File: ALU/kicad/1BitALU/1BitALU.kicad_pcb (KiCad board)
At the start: 2 copper layers, 165.1 x 165.1 mm, 55 parts, among them P1 CONN_6, P2 CONN_2, P3 Power, U1 xor3a, U10 and3a, U11 or2a, U12 and3b, U13 inv3b, U14 and3c, U15 or3a, U16 xor1b, U17 xor1a, U18 xor2b, U19 and4a, U2 and2a, U20 xor2a, U21 and4b, U22 and4c, U23 or3b, U24 and5a, U25 and5b, U26 inv5c, U27 and5c, U28 or3c, U29 and6a, U3 xor3b, U30 inv6b, U31 and6b, U32 inv6c, U33 and6c, U34 or3d, U4 and2b, U5 or1b, U6 and1a, U7 and1b, U8 or1a, U9 or2b

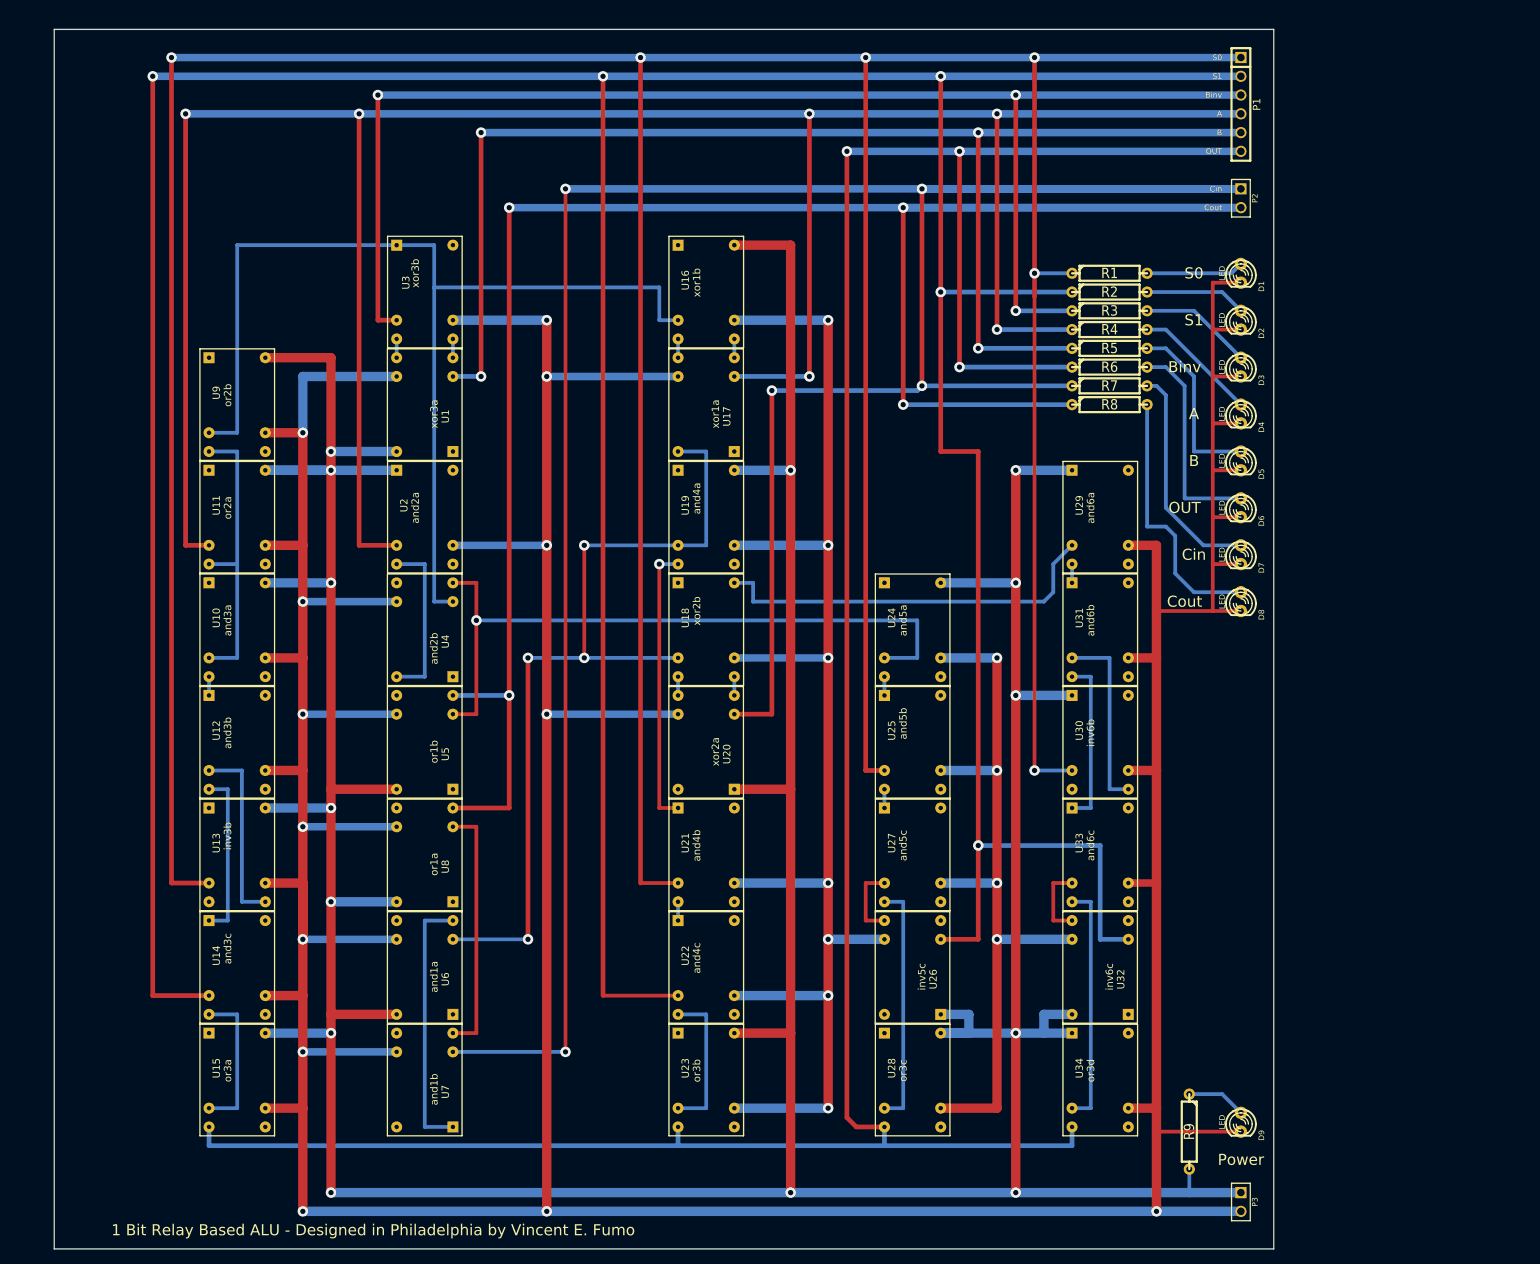
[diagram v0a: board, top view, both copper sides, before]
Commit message: * improvements
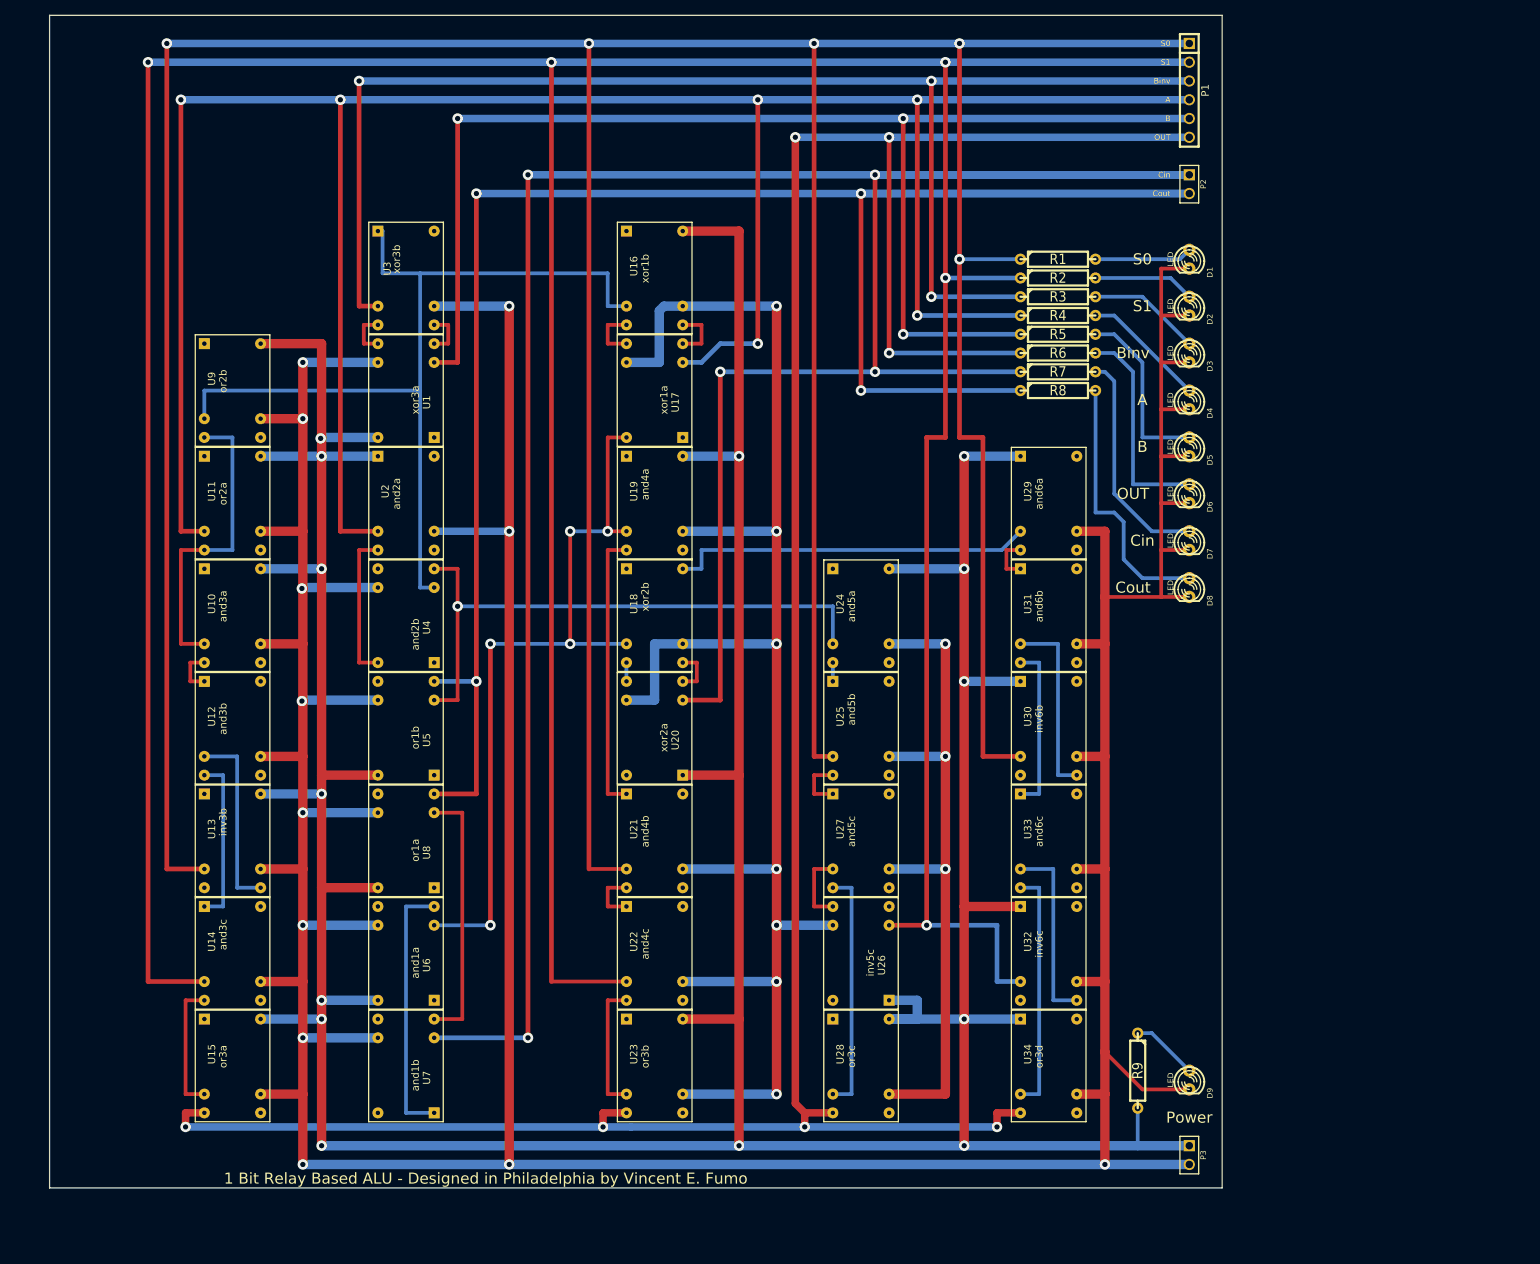
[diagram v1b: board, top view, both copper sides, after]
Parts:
- moved U32 14.6 mm to (156.8, 134.6), turned to 270 degrees
- moved R9 10.8 mm to (165.1, 156.8)
- moved P3 9.44 mm to (172.1, 168.3)
- moved D9 9.03 mm to (172.1, 158.1)
- moved U24 7.24 mm to (131.4, 88.9)
- moved U25 7.24 mm to (131.4, 104.1)
- moved U27 7.24 mm to (131.4, 119.4)
- moved U29 7.24 mm to (156.8, 73.7)
- moved U30 7.24 mm to (156.8, 104.1)
- moved U31 7.24 mm to (156.8, 88.9)
- moved U33 7.24 mm to (156.8, 119.4)
- moved U28 7.24 mm to (131.4, 149.9)
- moved U34 7.24 mm to (156.8, 149.9)
- moved U16 7.24 mm to (103.5, 43.2)
- moved U17 7.24 mm to (95.9, 71.1)
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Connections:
- U1 pad 1: (no net) -> Net-(U1-Pad1)
- U10 pad 1: (no net) -> Net-(U10-Pad1)
- U10 pad 7: (no net) -> Net-(U10-Pad7)
- U11 pad 1: (no net) -> Net-(U11-Pad1)
- U11 pad 7: (no net) -> Net-(U11-Pad7)
- U12 pad 12: (no net) -> Net-(U12-Pad12)
- U12 pad 7: (no net) -> Net-(U12-Pad7)
- U13 pad 1: (no net) -> Net-(U13-Pad1)
- U13 pad 6: (no net) -> Net-(U13-Pad6)
- U14 pad 12: (no net) -> Net-(U14-Pad12)
- U14 pad 7: (no net) -> Net-(U14-Pad7)
- U15 pad 1: (no net) -> Net-(U15-Pad1)
- U15 pad 7: (no net) -> Net-(U15-Pad7)
- U16 pad 1: (no net) -> Net-(U16-Pad1)
- U17 pad 1: (no net) -> Net-(U17-Pad1)
- U18 pad 1: (no net) -> Net-(U18-Pad1)
- U19 pad 1: (no net) -> Net-(U19-Pad1)
- U19 pad 7: (no net) -> Net-(U19-Pad7)
- U2 pad 12: (no net) -> Net-(U2-Pad12)
- U2 pad 7: (no net) -> Net-(U2-Pad7)
- U20 pad 12: (no net) -> Net-(U20-Pad12)
- U21 pad 12: (no net) -> Net-(U21-Pad12)
- U21 pad 7: (no net) -> Net-(U21-Pad7)
- U22 pad 12: (no net) -> Net-(U22-Pad12)
- U22 pad 7: (no net) -> Net-(U22-Pad7)
- U23 pad 1: (no net) -> Net-(U23-Pad1)
- U23 pad 7: (no net) -> Net-(U23-Pad7)
- U24 pad 1: (no net) -> Net-(U24-Pad1)
- U24 pad 7: (no net) -> Net-(U24-Pad7)
- U25 pad 12: (no net) -> Net-(U25-Pad12)
- U25 pad 7: (no net) -> Net-(U25-Pad7)
- U26 pad 12: (no net) -> Net-(U26-Pad12)
- U26 pad 6: (no net) -> Net-(U26-Pad6)
- U27 pad 12: (no net) -> Net-(U27-Pad12)
- U27 pad 7: (no net) -> Net-(U27-Pad7)
- U28 pad 1: (no net) -> Net-(U28-Pad1)
- U28 pad 7: (no net) -> Net-(U28-Pad7)
- U29 pad 12: (no net) -> Net-(U29-Pad12)
- U29 pad 7: (no net) -> Net-(U29-Pad7)
- U3 pad 12: (no net) -> Net-(U3-Pad12)
- U30 pad 12: (no net) -> Net-(U30-Pad12)
- U30 pad 6: (no net) -> Net-(U30-Pad6)
- U31 pad 12: (no net) -> Net-(U31-Pad12)
- U31 pad 7: (no net) -> Net-(U31-Pad7)
- U32 pad 1: (no net) -> +5V
- U32 pad 12: +5V -> Net-(U32-Pad12)
- U32 pad 6: (no net) -> Net-(U32-Pad6)
- U33 pad 12: (no net) -> Net-(U33-Pad12)
- U33 pad 7: (no net) -> Net-(U33-Pad7)
- U34 pad 12: (no net) -> Net-(U34-Pad12)
- U34 pad 7: (no net) -> Net-(U34-Pad7)
- U4 pad 1: (no net) -> Net-(U4-Pad1)
- U4 pad 7: (no net) -> Net-(U4-Pad7)
- U5 pad 1: (no net) -> Net-(U5-Pad1)
- U5 pad 7: (no net) -> Net-(U5-Pad7)
- U6 pad 1: (no net) -> Net-(U6-Pad1)
- U6 pad 7: (no net) -> Net-(U6-Pad7)
- U7 pad 12: (no net) -> Net-(U7-Pad12)
- U7 pad 7: (no net) -> Net-(U7-Pad7)
- U8 pad 1: (no net) -> Net-(U8-Pad1)
- U8 pad 7: (no net) -> Net-(U8-Pad7)
- U9 pad 1: (no net) -> Net-(U9-Pad1)
- U9 pad 7: (no net) -> Net-(U9-Pad7)
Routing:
- net GND: track 1040.1 -> 983.4 mm, vias 24 -> 22
- net +5V: track 653.4 -> 619.5 mm
- net S1 Bus: track 591.8 -> 562.6 mm
- net B Actual: track 144.1 -> 121.3 mm
- net Net-(U32-Pad7): track 10.2 -> 25.4 mm
- net XOR Out: track 116.8 -> 102.2 mm, vias 4 -> 5
- net AND Out: track 93.3 -> 80.0 mm
- net Cout: track 290.8 -> 281.9 mm
- net Net-(U25-Pad6): track 2.54 -> 7.62 mm
- net Net-(U21-Pad6): track 2.54 -> 7.62 mm
- net Net-(U16-Pad7): track 2.54 -> 7.62 mm
- net Net-(U16-Pad6): track 2.54 -> 7.62 mm
- net Cin: track 383.2 -> 378.5 mm
- net ADD Out: track 53.6 -> 49.3 mm
- net A: track 353.1 -> 349.0 mm
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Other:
- board size 165.1 x 165.1 mm -> 158.8 x 158.8 mm

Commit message: more updates
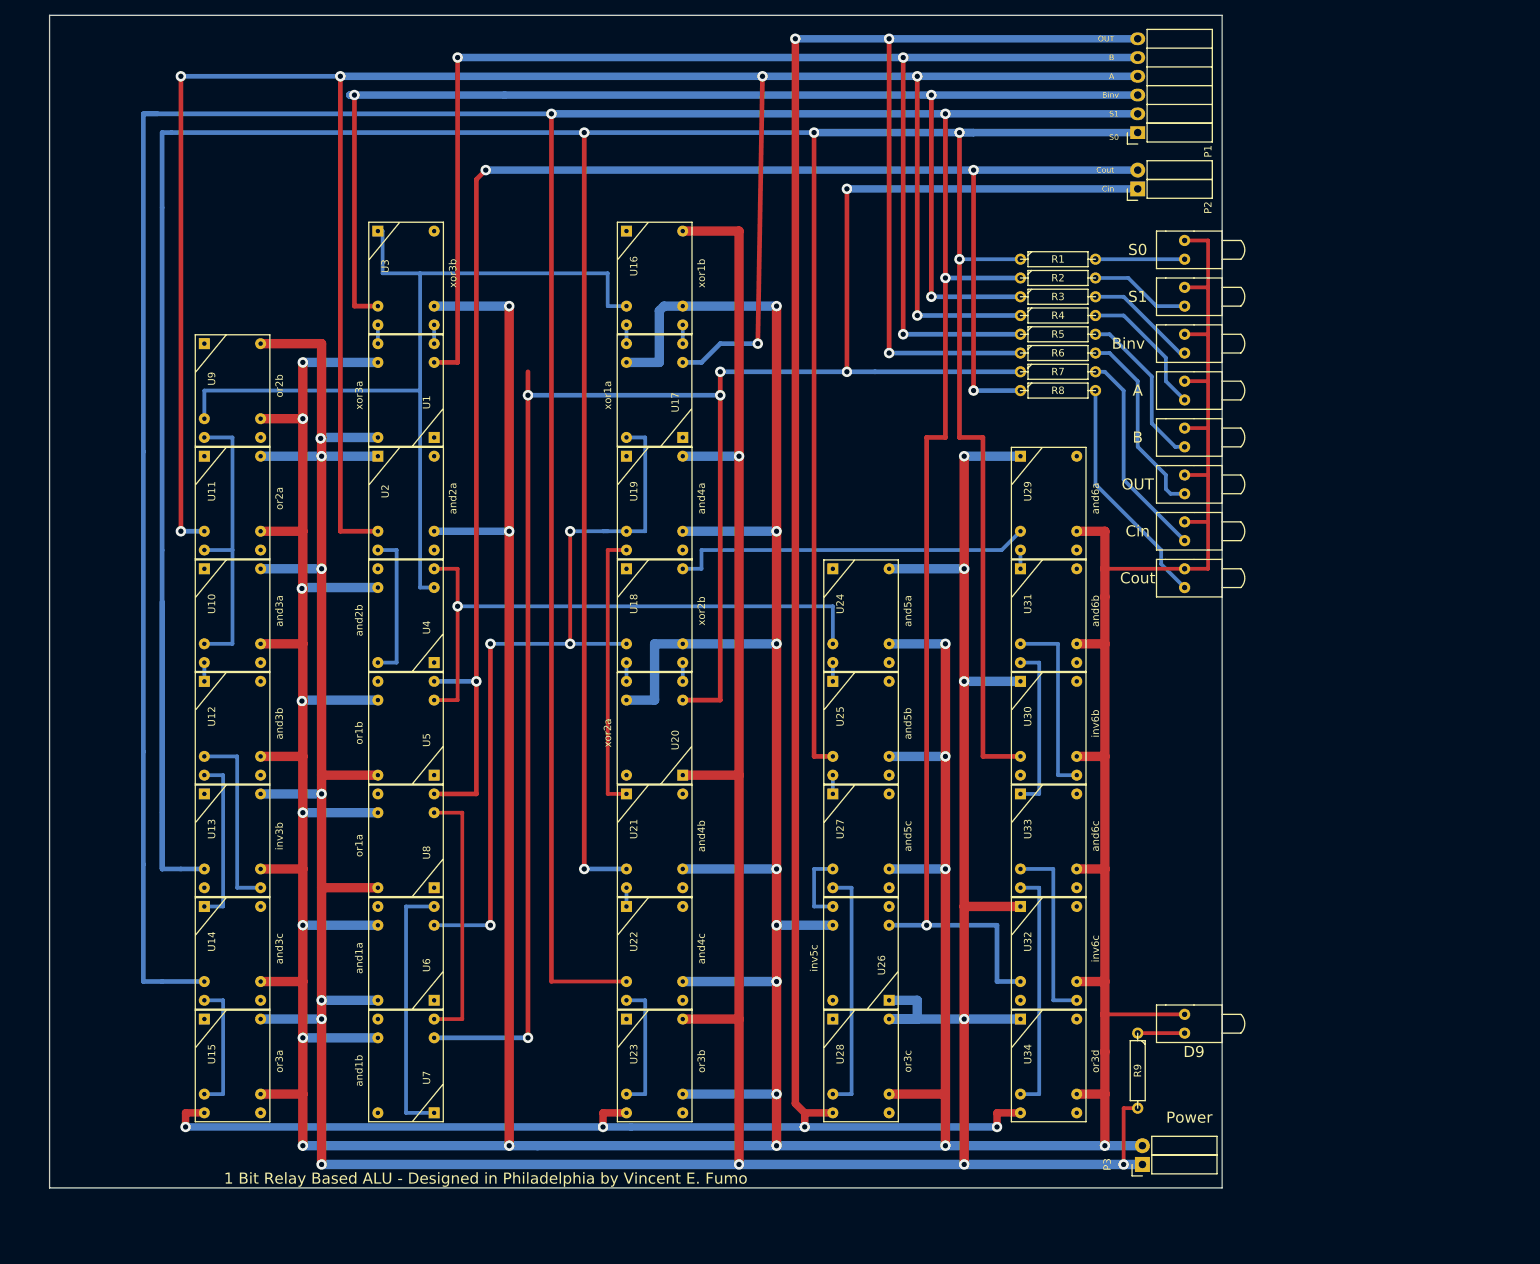
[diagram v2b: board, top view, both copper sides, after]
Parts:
- D1, D2, D3, D4, D5, D6, D7, D8, D9: footprint LED-3MM -> custom:90LED
- P1: footprint PIN_ARRAY-6X1 -> Socket_Strips:Socket_Strip_Angled_1x06
- P2, P3: footprint PIN_ARRAY_2X1 -> Socket_Strips:Socket_Strip_Angled_1x02
- R1, R2, R3, R4, R5, R6, R7, R8, R9: footprint R4 -> Discret:R4
- U1, U10, U11, U12, U13, U14, U15, U16, U17, U18, U19, U2, U20, U21, U22, U23, U24, U25, U26, U27, U28, U29, U3, U30, U31, U32, U33, U34, U4, U5, U6, U7, U8, U9: footprint 211ARelay -> custom:211ARelay
- moved D9 11.4 mm to (171.4, 146.7), turned to 0 degrees
- moved P1 9.03 mm to (165.1, 29.8), turned to 90 degrees
- moved P2 7.01 mm to (165.1, 37.5), turned to 90 degrees
- moved P3 6.48 mm to (165.7, 169.5), turned to 90 degrees
- moved D1 5.12 mm to (171.4, 41.9), turned to 0 degrees
- moved D2 5.12 mm to (171.4, 48.3), turned to 0 degrees
- moved D4 5.12 mm to (171.4, 61.0), turned to 0 degrees
- moved D3 5.12 mm to (171.4, 54.6), turned to 0 degrees
- moved D5 5.12 mm to (171.4, 67.3), turned to 0 degrees
- moved D6 5.12 mm to (171.4, 73.7), turned to 0 degrees
- moved D7 5.12 mm to (171.4, 80.0), turned to 0 degrees
- moved D8 5.12 mm to (171.4, 86.4), turned to 0 degrees
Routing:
- net Cin: track 378.5 -> 283.2 mm, vias 5 -> 6
- net GND: track 983.4 -> 1060.7 mm, vias 22 -> 24
- net Cout: track 281.9 -> 220.9 mm
- net S1 Bus: track 562.6 -> 537.8 mm, vias 5 -> 4
- net S0 Bus: track 584.2 -> 605.2 mm
- net OUT: track 363.1 -> 382.8 mm
- net B: track 180.3 -> 189.9 mm
- net Binv: track 186.7 -> 178.4 mm
- net A: track 349.0 -> 354.8 mm, vias 6 -> 7
- net +5V: track 619.5 -> 625.2 mm, vias 14 -> 15
- net Net-(U25-Pad6): track 7.62 -> 2.54 mm
- net Net-(U21-Pad6): track 7.62 -> 2.54 mm
- net Net-(U16-Pad7): track 7.62 -> 2.54 mm
- net Net-(U16-Pad6): track 7.62 -> 2.54 mm
- net Net-(D8-Pad1): track 35.9 -> 31.7 mm
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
